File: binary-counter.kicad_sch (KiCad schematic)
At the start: 5 parts, among them J1 Power, SW3 SW_SPDT, U22 74LS191

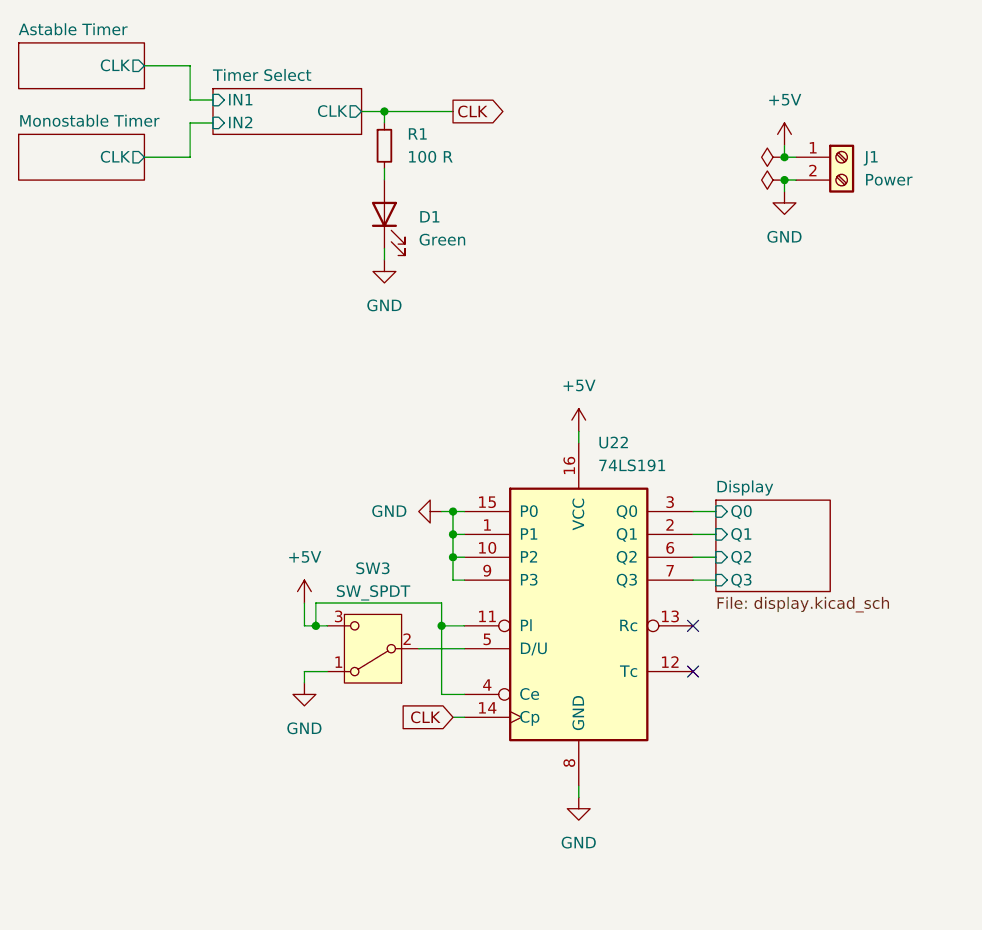
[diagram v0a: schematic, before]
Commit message: finished
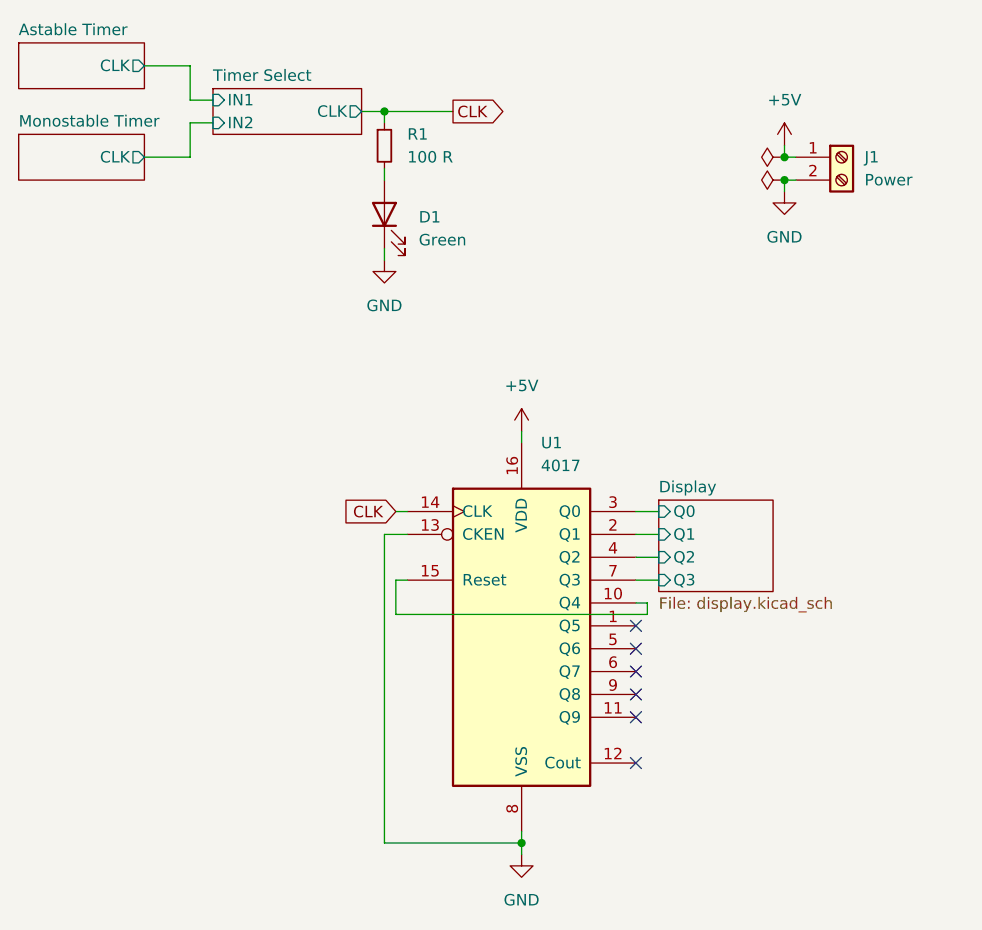
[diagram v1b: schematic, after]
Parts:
- removed SW3: SW_SPDT, Connector_PinHeader_1.27mm:PinHeader_1x03_P1.27mm_Vertical, symbol Switch:SW_SPDT
- removed U22: 74LS191, Package_DIP:DIP-16_W7.62mm_Socket, symbol 74xx:74LS191
- added U1: 4017, Package_DIP:DIP-16_W7.62mm_Socket, symbol 4xxx:4017
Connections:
- net +5V: now also U1.16 (VDD)
- net CLK: now also U1.14 (CLK)
- net Display/Q0: now also U1.3 (Q0)
- net Display/Q1: now also U1.2 (Q1)
- net Display/Q2: now also U1.4 (Q2)
- net Display/Q3: now also U1.7 (Q3)
- net GND: now also U1.13 (CKEN), U1.8 (VSS)
- new net: U1.10 (Q4), U1.15 (Reset)
- no-connect marks 2 -> 6
